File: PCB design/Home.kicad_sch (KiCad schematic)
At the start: 18 parts, among them J1 Fan, J2 LCD, J3 EM lock, J4 ACS712 Signal, J5 Power In, J7 RFID, J8 RFID, J9 LCD, K1 SANYOU_SRD_Form_C, U1 ACS712, U3 DHT11, U5 PIR, U6 MQ2

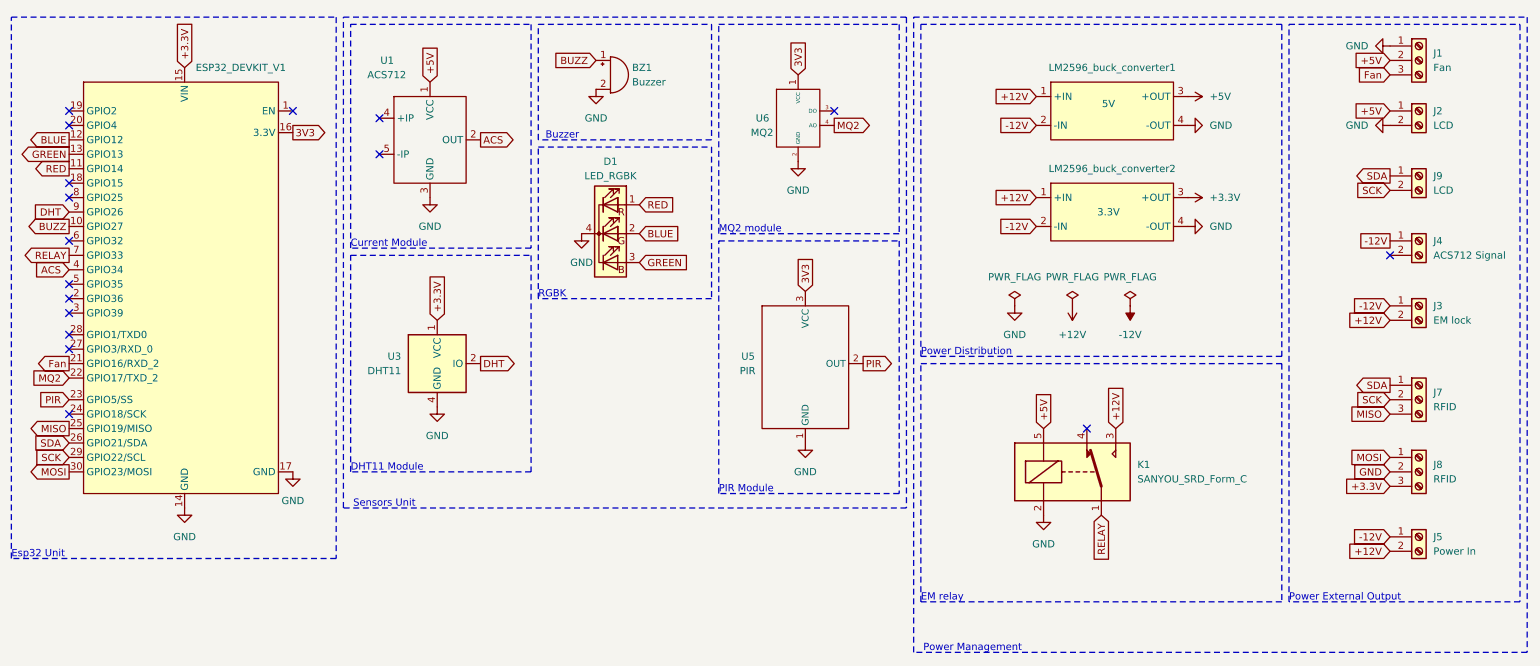
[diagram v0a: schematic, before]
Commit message: corrected plots
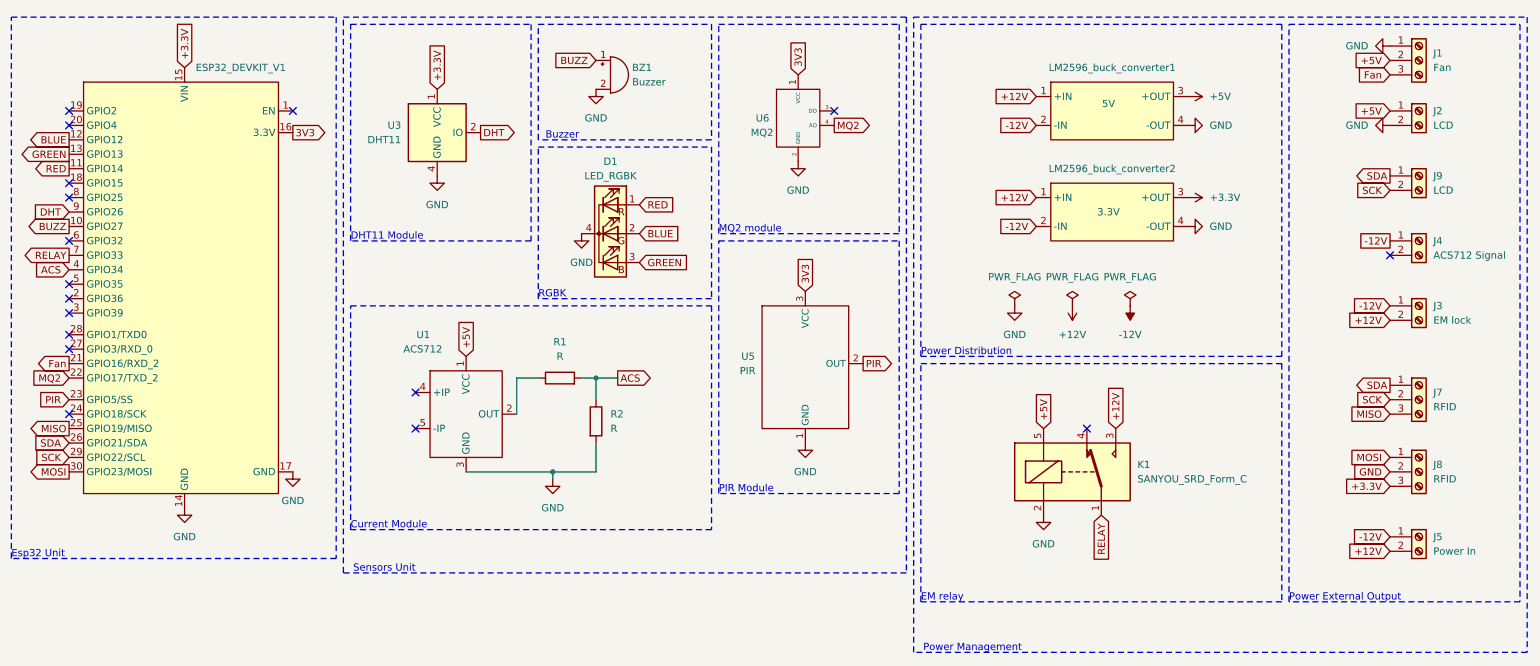
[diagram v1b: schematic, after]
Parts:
- added R1, R2: R, Resistor_THT:R_Axial_DIN0204_L3.6mm_D1.6mm_P5.08mm_Horizontal, symbol Device:R
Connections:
- net ACS: now also R1.2, R2.1; no longer U1.2 (OUT)
- net GND: now also R2.2
- new net: R1.1, U1.2 (OUT)
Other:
- moved on the sheet: U1, U3
